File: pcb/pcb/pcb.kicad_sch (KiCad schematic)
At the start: 27 parts, among them J1 SD Card, J2 Mic, J3 Relay Solenoid, J4 Status LED, SW1 Button Up, SW2 Button Down, SW3 Button Record, SW4 Button Delete, SW5 Button Play, U1 ESP32-C3-DevKitC-02

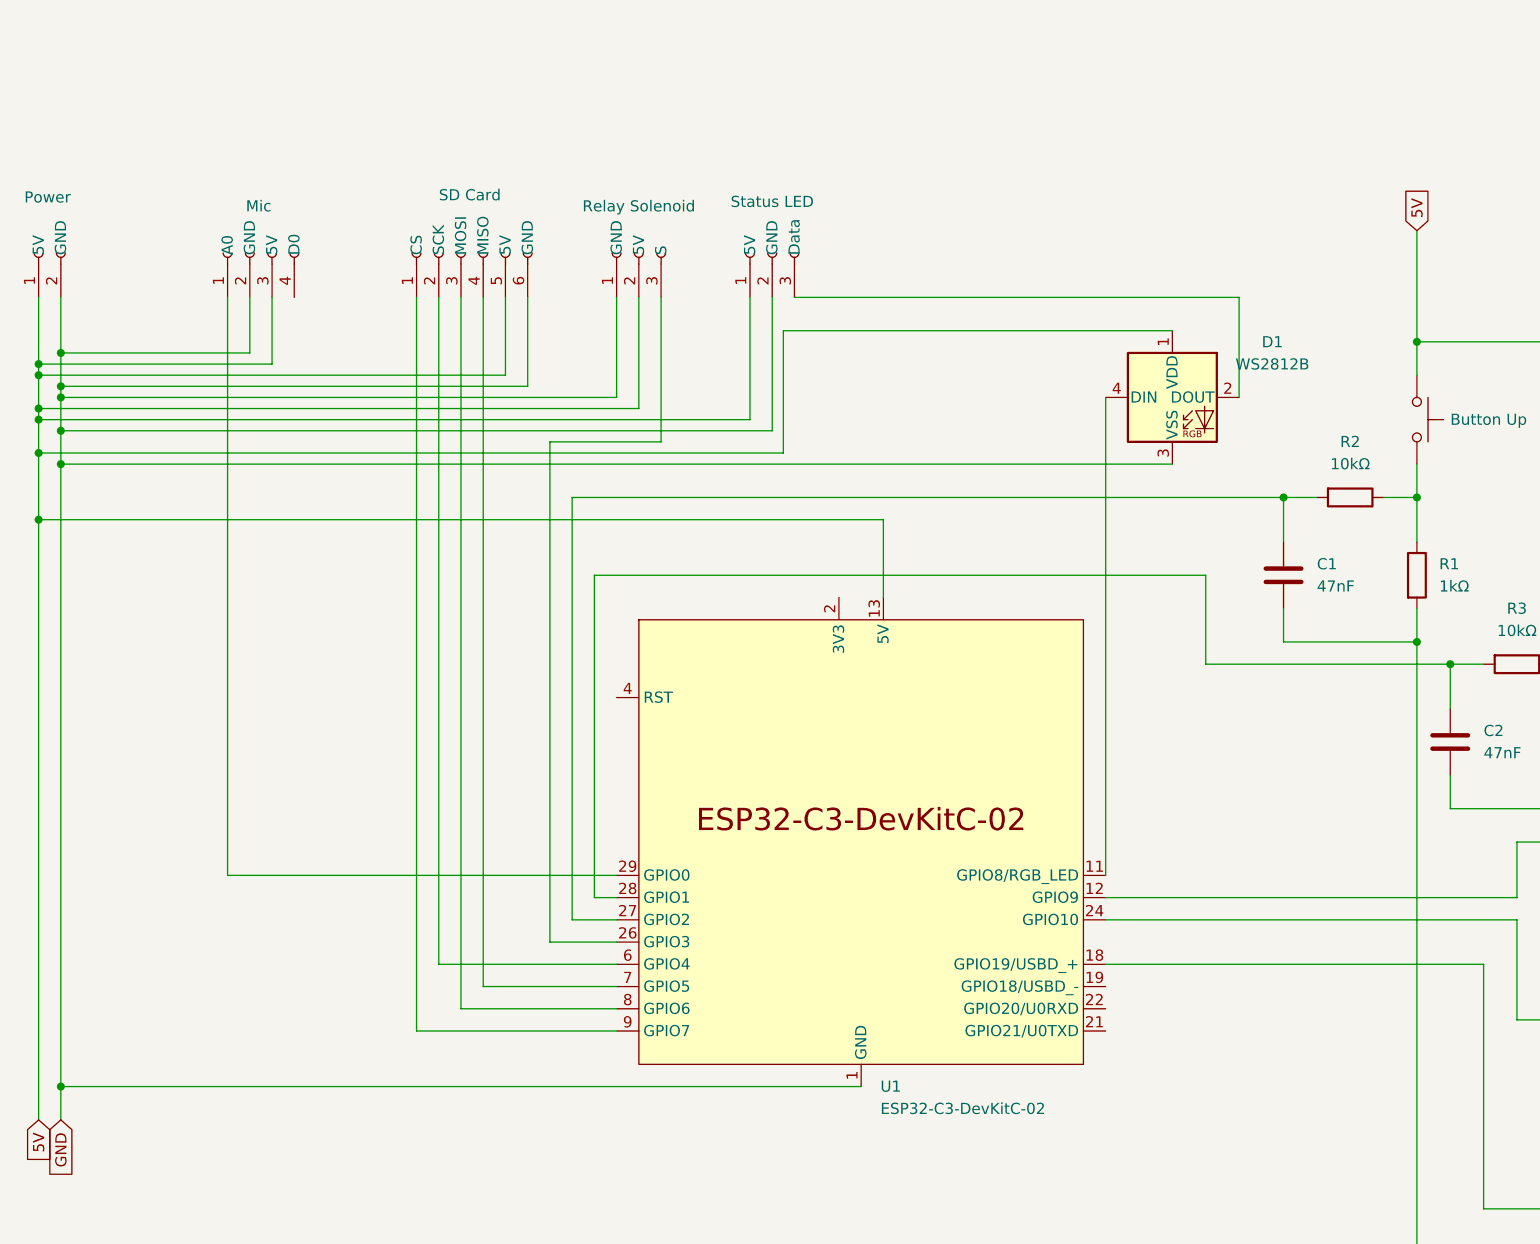
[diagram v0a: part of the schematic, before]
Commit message: update pcb
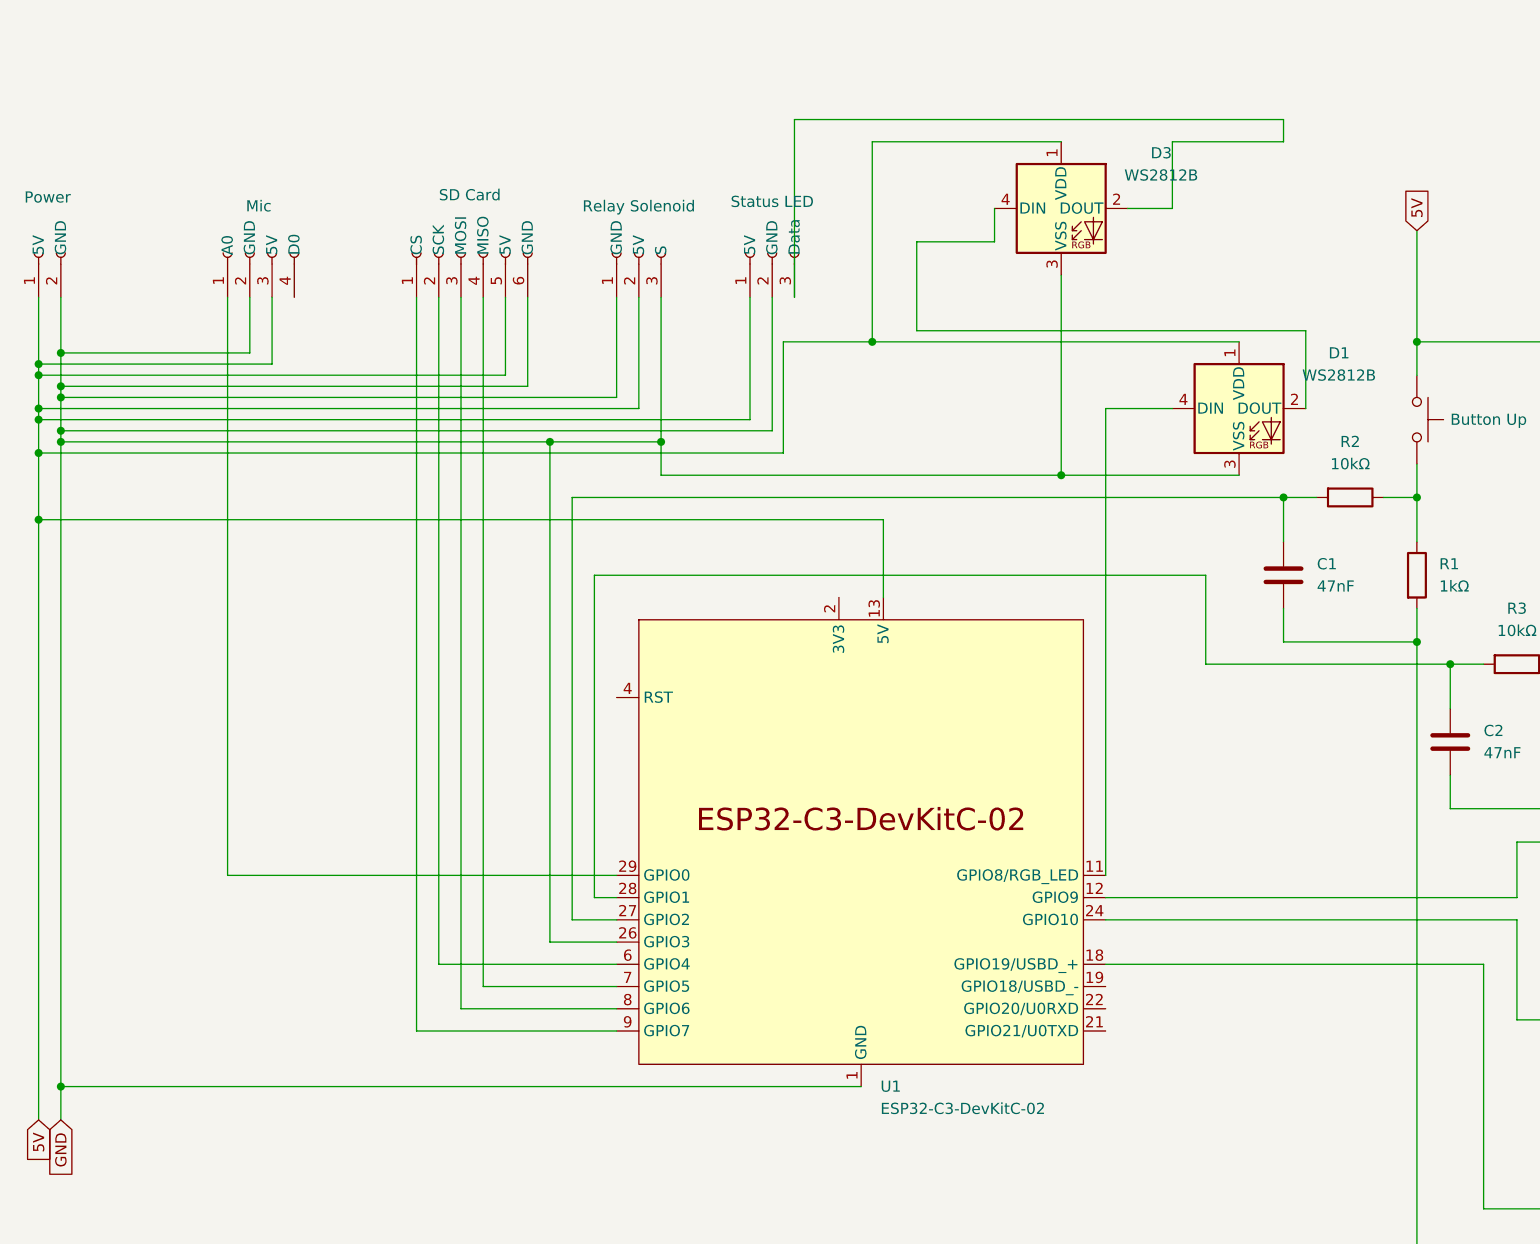
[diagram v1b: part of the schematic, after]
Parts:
- added D3: WS2812B, LED_SMD:LED_WS2812B_PLCC4_5.0x5.0mm_P3.2mm, symbol LED:WS2812B
- C1, C2, C3, C4, C5: footprint (none) -> Capacitor_THT:C_Disc_D5.0mm_W2.5mm_P5.00mm
- R1, R10, R2, R3, R4, R5, R6, R7, R8, R9: footprint (none) -> Resistor_THT:R_Axial_DIN0207_L6.3mm_D2.5mm_P15.24mm_Horizontal
- SW1, SW2, SW3, SW4, SW5: footprint (none) -> Button_Switch_SMD:SW_SPST_Omron_B3FS-101xP
- renumbered P to P1
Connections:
- net 5V: now also D3.1 (VDD)
- net GND: now also J3.3 (S), U1.26 (GPIO3), D3.3 (VSS)
- net at D1.2 (DOUT): now also D3.4 (DIN); no longer J4.3 (Data)
- new net: D3.2 (DOUT), J4.3 (Data)
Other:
- moved on the sheet: D1

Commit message: update
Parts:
- D3: footprint LED_SMD:LED_WS2812B_PLCC4_5.0x5.0mm_P3.2mm -> (none)
- R1, R10, R2, R3, R4, R5, R6, R7, R8, R9: footprint Resistor_THT:R_Axial_DIN0207_L6.3mm_D2.5mm_P15.24mm_Horizontal -> Resistor_THT:R_Axial_DIN0207_L6.3mm_D2.5mm_P10.16mm_Horizontal
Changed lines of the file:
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@@
 			)
 		)
-		(property "Footprint" "Resistor_THT:R_Axial_DIN0207_L6.3mm_D2.5mm_P15.24mm_Horizontal"
+		(property "Footprint" "Resistor_THT:R_Axial_DIN0207_L6.3mm_D2.5mm_P10.16mm_Horizontal"
 			(at 244.602 128.27 90)
 			(effects
@@
 			)
 		)
-		(property "Footprint" "Resistor_THT:R_Axial_DIN0207_L6.3mm_D2.5mm_P15.24mm_Horizontal"
+		(property "Footprint" "Resistor_THT:R_Axial_DIN0207_L6.3mm_D2.5mm_P10.16mm_Horizontal"
 			(at 180.34 57.912 90)
 			(effects
@@
 			)
 		)
-		(property "Footprint" "Resistor_THT:R_Axial_DIN0207_L6.3mm_D2.5mm_P15.24mm_Horizontal"
+		(property "Footprint" "Resistor_THT:R_Axial_DIN0207_L6.3mm_D2.5mm_P10.16mm_Horizontal"
 			(at 264.922 149.86 90)
 			(effects
@@
 			)
 		)
-		(property "Footprint" "Resistor_THT:R_Axial_DIN0207_L6.3mm_D2.5mm_P15.24mm_Horizontal"
+		(property "Footprint" "Resistor_THT:R_Axial_DIN0207_L6.3mm_D2.5mm_P10.16mm_Horizontal"
 			(at 205.232 87.63 90)
 			(effects
@@
 			)
 		)
-		(property "Footprint" "Resistor_THT:R_Axial_DIN0207_L6.3mm_D2.5mm_P15.24mm_Horizontal"
+		(property "Footprint" "Resistor_THT:R_Axial_DIN0207_L6.3mm_D2.5mm_P10.16mm_Horizontal"
 			(at 238.76 117.602 90)
 			(effects
@@
 			)
 		)
-		(property "Footprint" "Resistor_THT:R_Axial_DIN0207_L6.3mm_D2.5mm_P15.24mm_Horizontal"
+		(property "Footprint" "Resistor_THT:R_Axial_DIN0207_L6.3mm_D2.5mm_P10.16mm_Horizontal"
 			(at 224.282 107.95 90)
 			(effects
@@
 			)
 		)
-		(property "Footprint" "Resistor_THT:R_Axial_DIN0207_L6.3mm_D2.5mm_P15.24mm_Horizontal"
+		(property "Footprint" "Resistor_THT:R_Axial_DIN0207_L6.3mm_D2.5mm_P10.16mm_Horizontal"
 			(at 259.08 139.192 90)
 			(effects
@@
 			)
 		)
-		(property "Footprint" "Resistor_THT:R_Axial_DIN0207_L6.3mm_D2.5mm_P15.24mm_Horizontal"
+		(property "Footprint" "Resistor_THT:R_Axial_DIN0207_L6.3mm_D2.5mm_P10.16mm_Horizontal"
 			(at 186.182 68.58 90)
 			(effects
@@
 			)
 		)
-		(property "Footprint" "Resistor_THT:R_Axial_DIN0207_L6.3mm_D2.5mm_P15.24mm_Horizontal"
+		(property "Footprint" "Resistor_THT:R_Axial_DIN0207_L6.3mm_D2.5mm_P10.16mm_Horizontal"
 			(at 199.39 76.962 90)
 			(effects
@@
 			)
 		)
-		(property "Footprint" "LED_SMD:LED_WS2812B_PLCC4_5.0x5.0mm_P3.2mm"
+		(property "Footprint" ""
 			(at 148.59 34.29 0)
 			(effects
@@
 			)
 		)
-		(property "Footprint" "Resistor_THT:R_Axial_DIN0207_L6.3mm_D2.5mm_P15.24mm_Horizontal"
+		(property "Footprint" "Resistor_THT:R_Axial_DIN0207_L6.3mm_D2.5mm_P10.16mm_Horizontal"
 			(at 218.44 97.282 90)
 			(effects

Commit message: Final_PCB
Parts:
- J1: footprint (none) -> TerminalBlock:TerminalBlock_MaiXu_MX126-5.0-06P_1x06_P5.00mm
- J2: footprint (none) -> TerminalBlock:TerminalBlock_MaiXu_MX126-5.0-04P_1x04_P5.00mm
- J3, J4: footprint (none) -> TerminalBlock:TerminalBlock_bornier-3_P5.08mm
- P1: footprint (none) -> TerminalBlock:TerminalBlock_bornier-2_P5.08mm
- SW1, SW2, SW3, SW4, SW5: footprint Button_Switch_SMD:SW_SPST_Omron_B3FS-101xP -> Button_Switch_THT:SW_PUSH_6mm_H4.3mm
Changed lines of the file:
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@@
 			)
 		)
-		(property "Footprint" ""
+		(property "Footprint" "TerminalBlock:TerminalBlock_MaiXu_MX126-5.0-04P_1x04_P5.00mm"
 			(at 54.61 31.75 0)
 			(effects
@@
 			)
 		)
-		(property "Footprint" ""
+		(property "Footprint" "TerminalBlock:TerminalBlock_bornier-2_P5.08mm"
 			(at 30.48 31.75 0)
 			(effects
@@
 			)
 		)
-		(property "Footprint" ""
+		(property "Footprint" "TerminalBlock:TerminalBlock_MaiXu_MX126-5.0-06P_1x06_P5.00mm"
 			(at 78.74 31.75 0)
 			(effects
@@
 			)
 		)
-		(property "Footprint" "Button_Switch_SMD:SW_SPST_Omron_B3FS-101xP"
+		(property "Footprint" "Button_Switch_THT:SW_PUSH_6mm_H4.3mm"
 			(at 193.04 50.8 0)
 			(effects
@@
 			)
 		)
-		(property "Footprint" "Button_Switch_SMD:SW_SPST_Omron_B3FS-101xP"
+		(property "Footprint" "Button_Switch_THT:SW_PUSH_6mm_H4.3mm"
 			(at 271.78 50.8 0)
 			(effects
@@
 			)
 		)
-		(property "Footprint" "Button_Switch_SMD:SW_SPST_Omron_B3FS-101xP"
+		(property "Footprint" "Button_Switch_THT:SW_PUSH_6mm_H4.3mm"
 			(at 212.09 50.8 0)
 			(effects
@@
 			)
 		)
-		(property "Footprint" ""
+		(property "Footprint" "TerminalBlock:TerminalBlock_bornier-3_P5.08mm"
 			(at 114.3 31.75 0)
 			(effects
@@
 			)
 		)
-		(property "Footprint" "Button_Switch_SMD:SW_SPST_Omron_B3FS-101xP"
+		(property "Footprint" "Button_Switch_THT:SW_PUSH_6mm_H4.3mm"
 			(at 251.46 50.8 0)
 			(effects
@@
 			)
 		)
-		(property "Footprint" "Button_Switch_SMD:SW_SPST_Omron_B3FS-101xP"
+		(property "Footprint" "Button_Switch_THT:SW_PUSH_6mm_H4.3mm"
 			(at 231.14 50.8 0)
 			(effects
@@
 			)
 		)
-		(property "Footprint" ""
+		(property "Footprint" "TerminalBlock:TerminalBlock_bornier-3_P5.08mm"
 			(at 99.06 31.75 0)
 			(effects
